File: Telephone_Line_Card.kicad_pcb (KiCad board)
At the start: 2 copper layers, 101.6 x 88.9 mm, 36 parts, among them J1 Conn_01x12, J2 RJ11, K1 TELTONE_M949-1, K2 G5V-2, Q1 2N3904, T1 600:600, U1 4N35

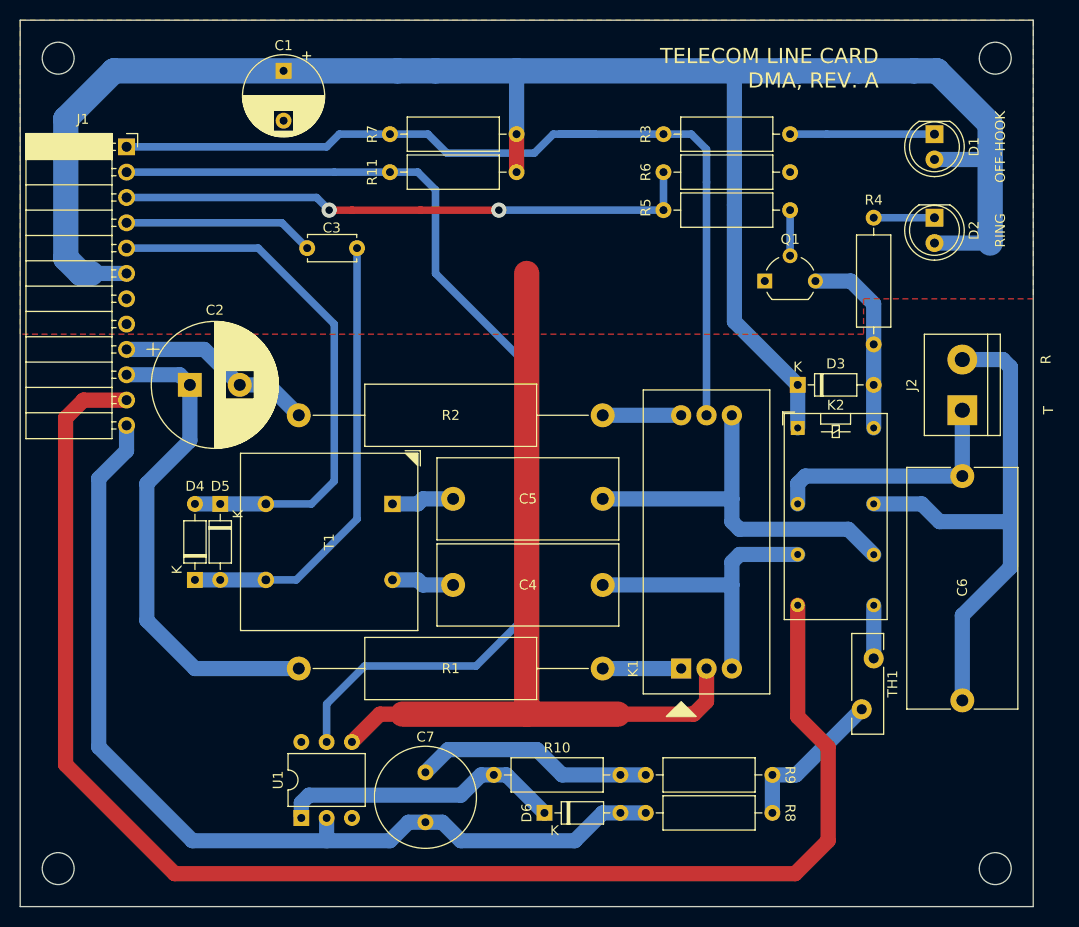
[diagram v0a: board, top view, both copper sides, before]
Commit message: generated gerbers
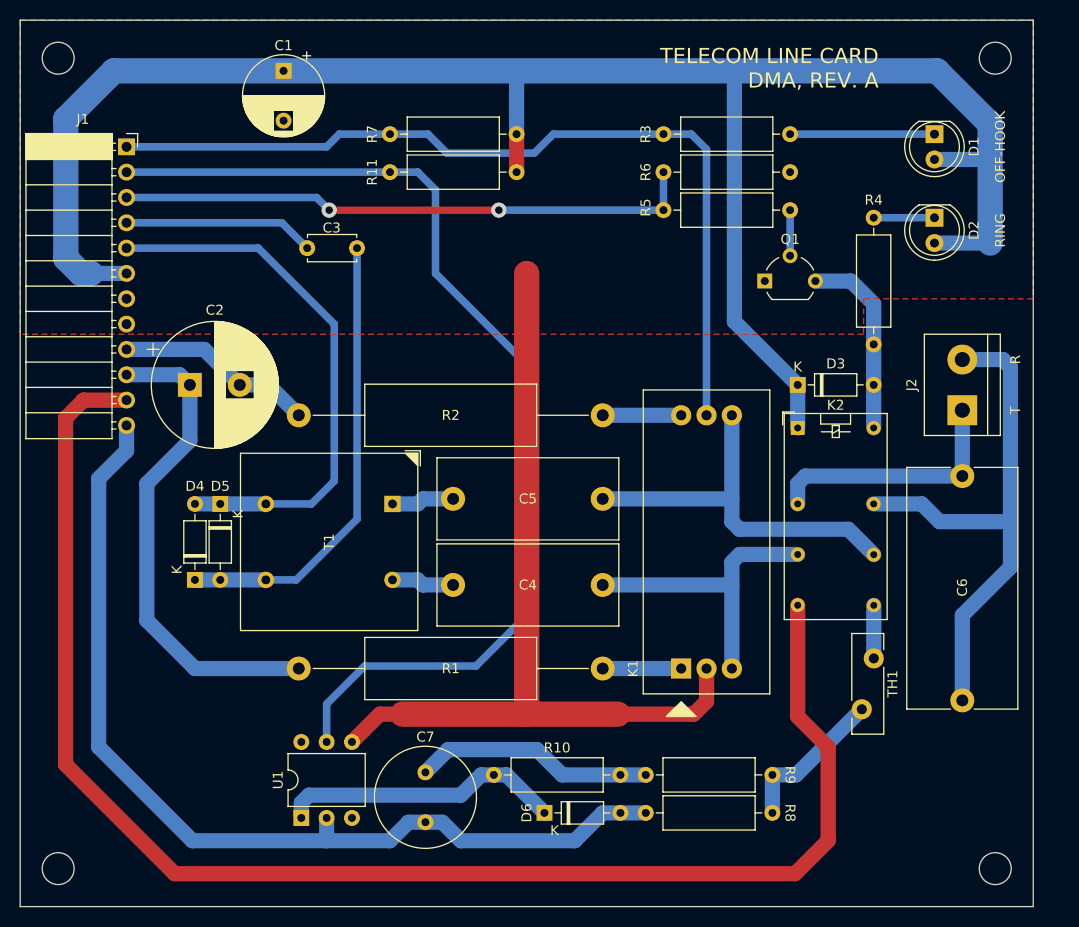
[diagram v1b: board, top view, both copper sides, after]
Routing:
- net SHK: track 91.4 -> 87.6 mm
